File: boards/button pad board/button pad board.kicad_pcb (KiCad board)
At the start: 2 copper layers, 200 x 55.2 mm, 22 parts, among them J1 RGB, J2 INPUTS

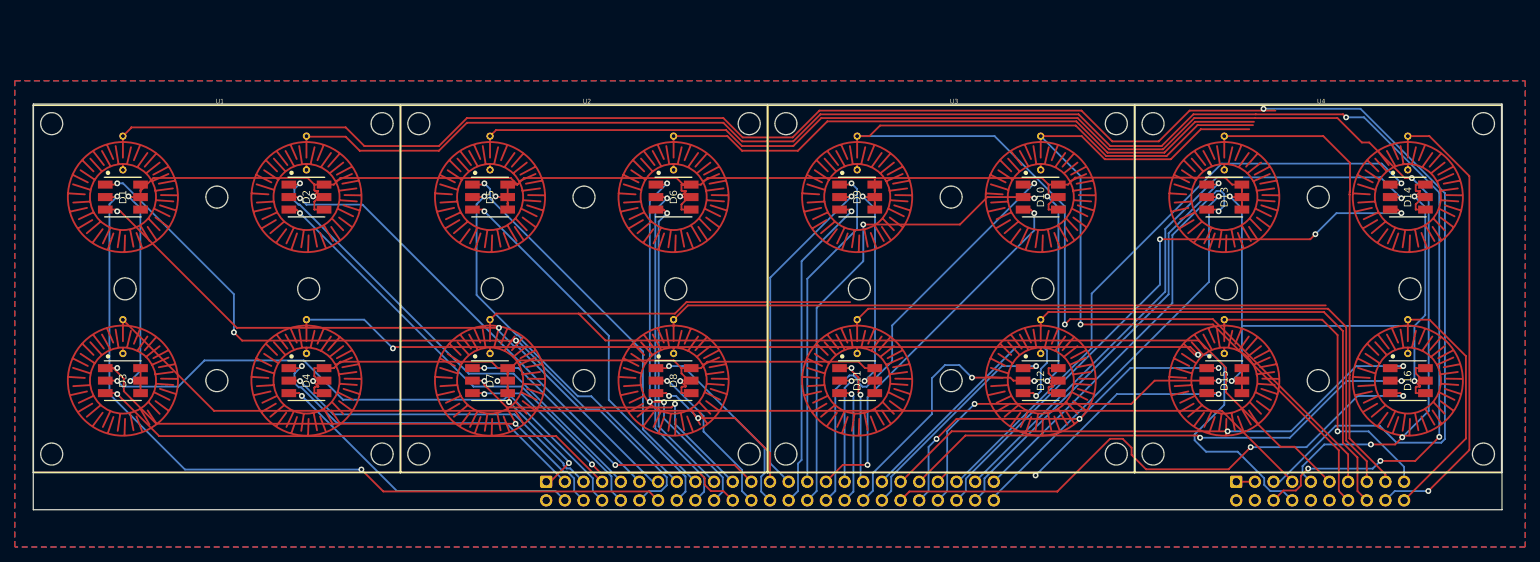
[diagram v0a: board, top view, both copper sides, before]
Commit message: button board updated, routed, and ready to rock.
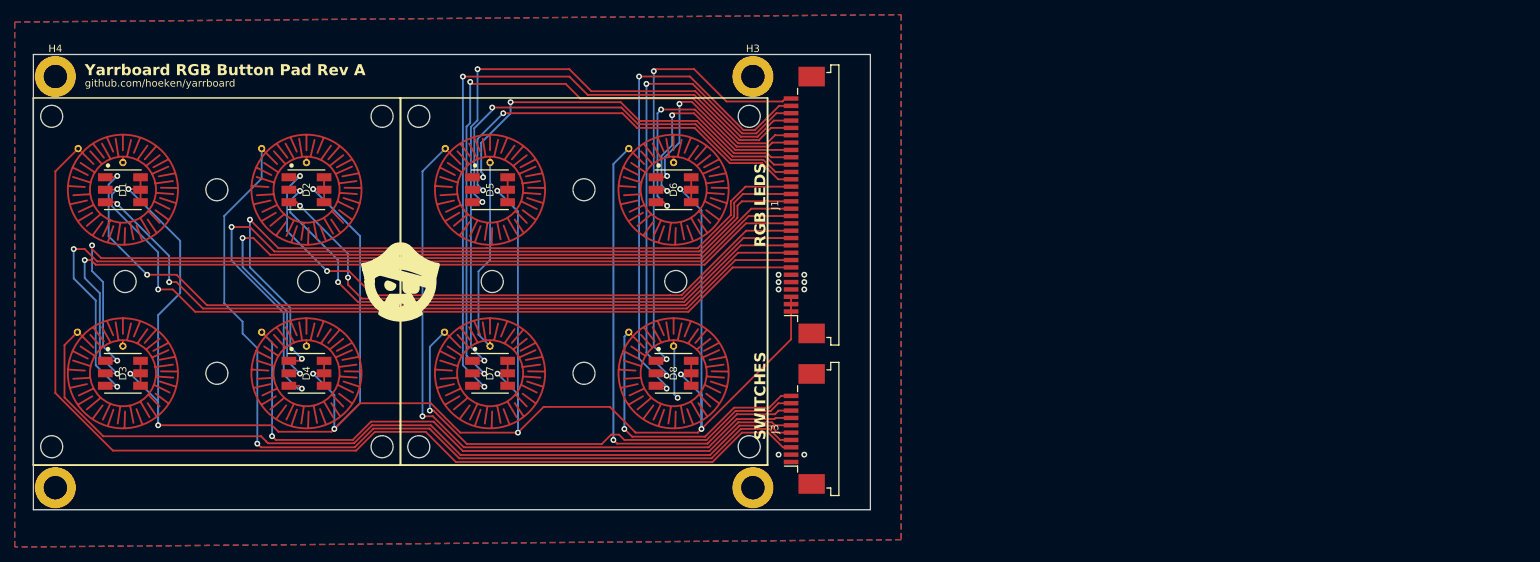
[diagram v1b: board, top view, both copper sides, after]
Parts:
- removed D10, D11, D12, D13, D14, D15, D16, D9: LED_RBGA, yarrboard:WURTH_LED_RGB_5050-6
- removed J2: INPUTS, Connector_IDC:IDC-Header_2x10_P2.54mm_Horizontal
- removed U3, U4: ~, yarrboard:BUTTONPAD-2X2
- added H1: MountingHole, MountingHole:MountingHole_3.2mm_M3_DIN965_Pad, F.Cu at (143.7, 93.5)
- added H2: MountingHole, MountingHole:MountingHole_3.2mm_M3_DIN965_Pad, F.Cu at (48.7, 93.5)
- added H3: MountingHole, MountingHole:MountingHole_3.2mm_M3_DIN965_Pad, F.Cu at (143.7, 37.5)
- added H4: MountingHole, MountingHole:MountingHole_3.2mm_M3_DIN965_Pad, F.Cu at (48.7, 37.5)
- added J3: INPUTS, Connector_FFC-FPC:TE_1-84952-0_1x10-1MP_P1.0mm_Horizontal, F.Cu at (150.7, 85.5)
- added REF**: Logo Small, yarrboard:Logo Small, F.Cu at (95.7, 65.5)
- J1: footprint Connector_IDC:IDC-Header_2x25_P2.54mm_Horizontal -> Connector_FFC-FPC:TE_3-84952-0_1x30-1MP_P1.0mm_Horizontal; moved to F.Cu
- moved J1 51.5 mm to (150.7, 55.0), turned to 90 degrees
- moved D1 1.00 mm to (57.9, 52.9)
- moved D2 1.00 mm to (82.9, 52.9)
- moved D3 1.00 mm to (57.9, 77.9)
- moved D4 1.00 mm to (82.9, 77.9)
- moved D5 1.00 mm to (107.9, 52.9)
- moved D6 1.00 mm to (132.9, 52.9)
- moved D7 1.00 mm to (107.9, 77.9)
- moved D8 1.00 mm to (132.9, 77.9)
- moved U1 1.00 mm to (45.7, 90.4)
- moved U2 1.00 mm to (95.7, 90.4)
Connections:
- J1 pad 10: G1 -> R1
- J1 pad 11: R1 -> G1
- J1 pad 12: B0 -> B1
- J1 pad 13: G0 -> R2
- J1 pad 14: R0 -> G2
- J1 pad 15: R4 -> B2
- J1 pad 16: G4 -> R3
- J1 pad 17: B4 -> G3
- J1 pad 18: R5 -> B3
- J1 pad 19: G5 -> R4
- J1 pad 2: GND -> +5V
- J1 pad 20: B5 -> G4
- J1 pad 21: R6 -> B4
- J1 pad 22: G6 -> R5
- J1 pad 23: B6 -> G5
- J1 pad 24: R7 -> B5
- J1 pad 25: G7 -> R6
- J1 pad 26: B7 -> G6
- J1 pad 27: R8 -> B6
- J1 pad 28: G8 -> R7
- J1 pad 29: B8 -> G7
- J1 pad 3: B3 -> +5V
- J1 pad 30: R9 -> B7
- J1 pad 4: G3 -> GND
- J1 pad 5: R3 -> GND
- J1 pad 6: B2 -> GND
- J1 pad 7: G2 -> R0
- J1 pad 8: R2 -> G0
- J1 pad 9: B1 -> B0
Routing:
- net +5V: track 521.7 -> 320.5 mm, vias 18 -> 12
- net SW8: track 156.5 -> 0.00 mm, vias 1 -> 0
- net SW0: track 257.1 -> 143.3 mm, vias 1 -> 0
- net SW9: track 108.9 -> 0.00 mm, vias 1 -> 0
- net SW1: track 227.4 -> 122.1 mm, vias 4 -> 1
- net SW4: track 190.8 -> 91.3 mm, vias 3 -> 1
- net SW6: track 163.8 -> 65.5 mm, vias 0 -> 1
- net SW10: track 90.5 -> 0.00 mm
- net B13: track 85.6 -> 0.00 mm, vias 1 -> 0
- net G13: track 83.1 -> 0.00 mm, vias 3 -> 0
- net R13: track 83.0 -> 0.00 mm, vias 1 -> 0
- net G15: track 80.3 -> 0.00 mm, vias 2 -> 0
- net B15: track 76.9 -> 0.00 mm, vias 2 -> 0
- net R15: track 73.2 -> 0.00 mm, vias 2 -> 0
- net SW11: track 67.1 -> 0.00 mm
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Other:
- board size 200 x 55.2 mm -> 114 x 62 mm
- board text added: "RGB LEDS"
- board text added: "SWITCHES"
- board text added: "Yarrboard RGB Button Pad Rev A"
- board text added: "github.com/hoeken/yarrboard"
